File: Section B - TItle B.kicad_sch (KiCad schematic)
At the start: 3 parts, among them IC2 TPS61086DRCR

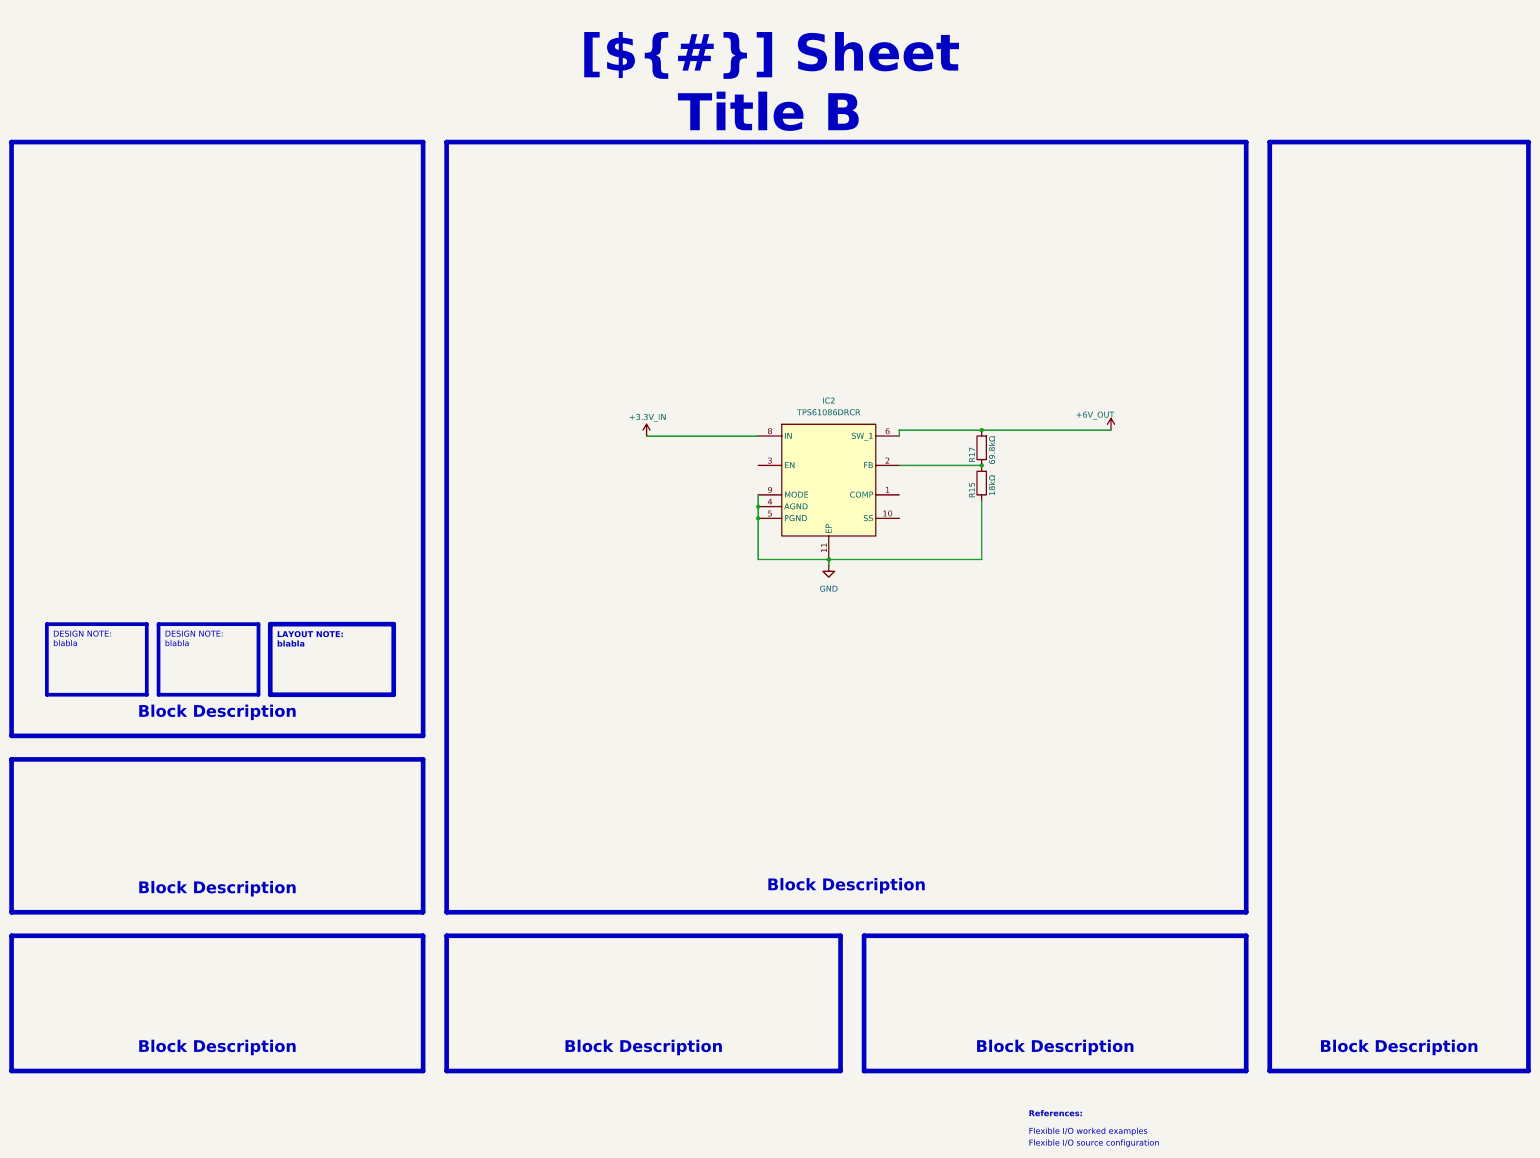
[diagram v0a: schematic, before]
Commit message: [Finish schématique]
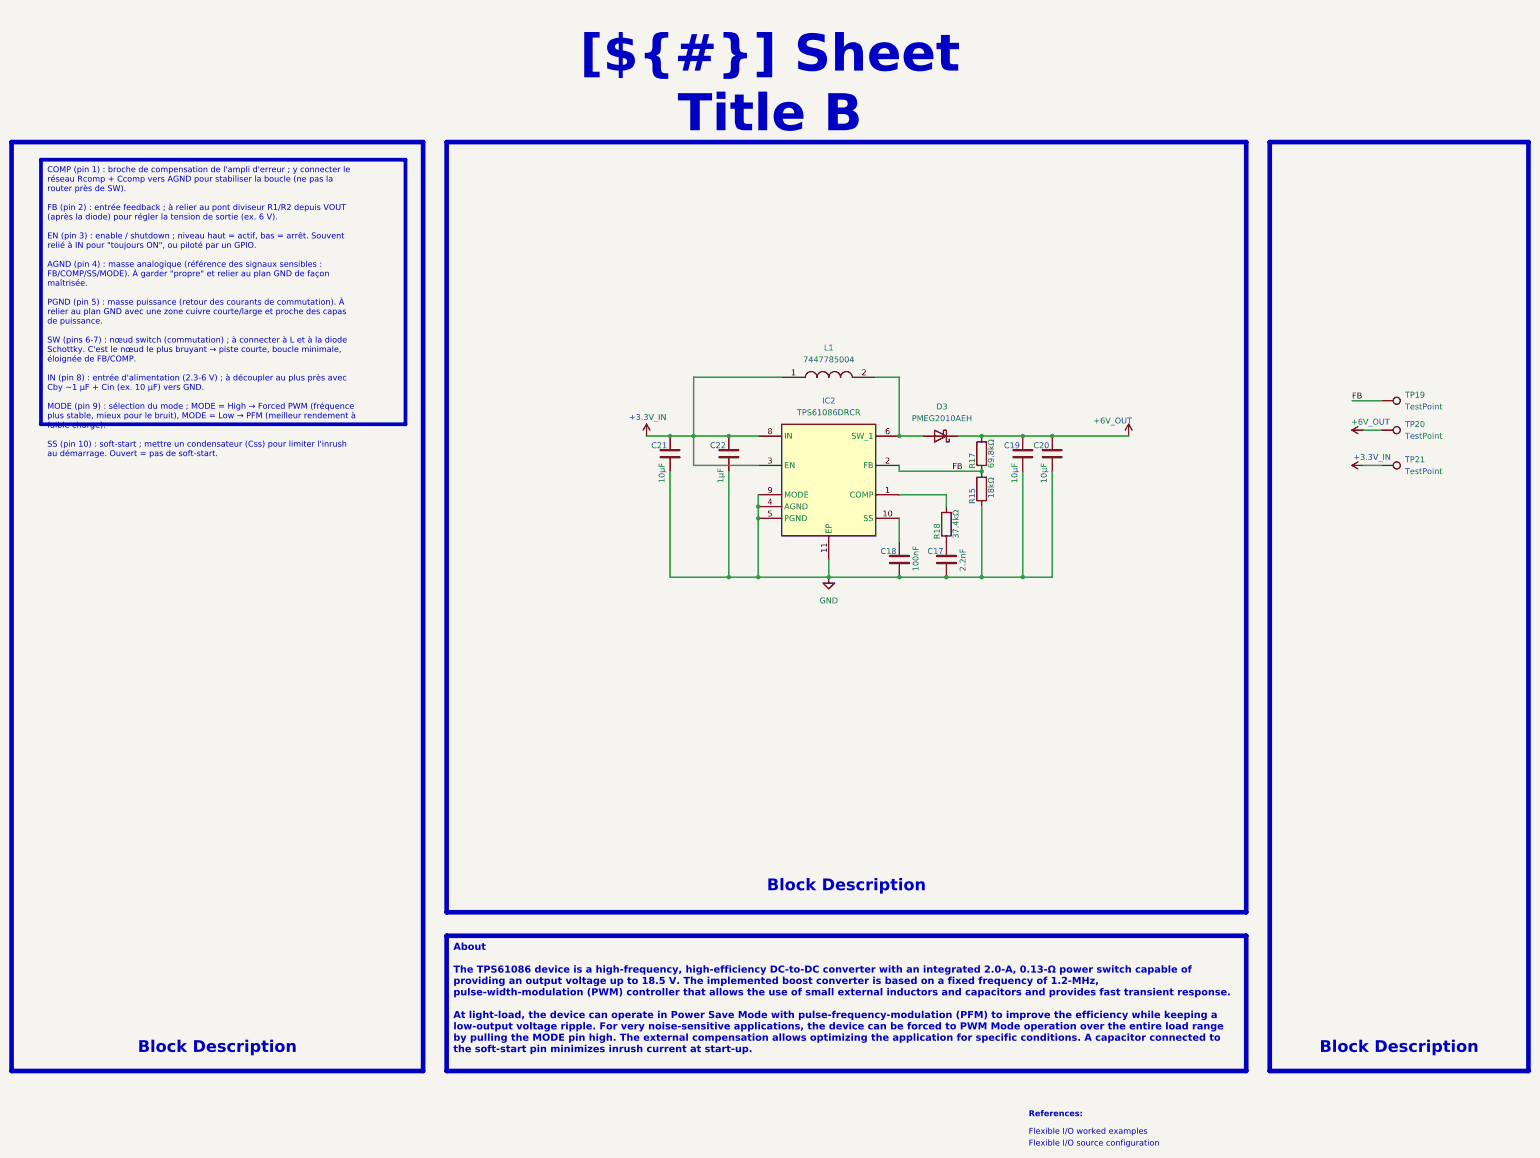
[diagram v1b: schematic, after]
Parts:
- added C17: 2.2nF, Capacitor_SMD:C_0603_1608Metric, symbol Device:C
- added C18: 100nF, Capacitor_SMD:C_0603_1608Metric, symbol Device:C
- added C19, C20, C21: 10µF, Capacitor_SMD:C_0603_1608Metric, symbol Device:C
- added C22: 1µF, Capacitor_SMD:C_0603_1608Metric, symbol Device:C
- added D3: PMEG2010AEH, Diode_SMD:D_SOD-123F, symbol Diode:PMEG2010AEH
- added L1: 7447785004, 7447785004, symbol 7447785004:7447785004
- added R18: 37.4kΩ, Resistor_SMD:R_0603_1608Metric, symbol Device:R
- added TP19, TP20, TP21: TestPoint, TestPoint:TestPoint_Pad_D2.0mm, symbol Connector:TestPoint
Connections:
- net +3.3V_IN: now also IC2.3 (EN), C21.1, C22.1, L1.1, TP21.1
- net +6V_OUT: now also C19.1, C20.1, D3.1 (K), TP20.1; no longer IC2.6 (SW_1), IC2.7 (SW_2)
- net GND: now also C17.2, C18.2, C19.2, C20.2, C21.2, C22.2
- net at IC2.1 (COMP): now also R18.2
- net at IC2.10 (SS): now also C18.1
- net FB: now reaches IC2.2 (FB), R15.2, R17.1
- net FB: now also TP19.1
- new net: C17.1, R18.1
- new net: D3.2 (A), IC2.6 (SW_1), IC2.7 (SW_2), L1.2
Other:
- moved on the sheet: R15, R17

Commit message: [Finish schématiq]
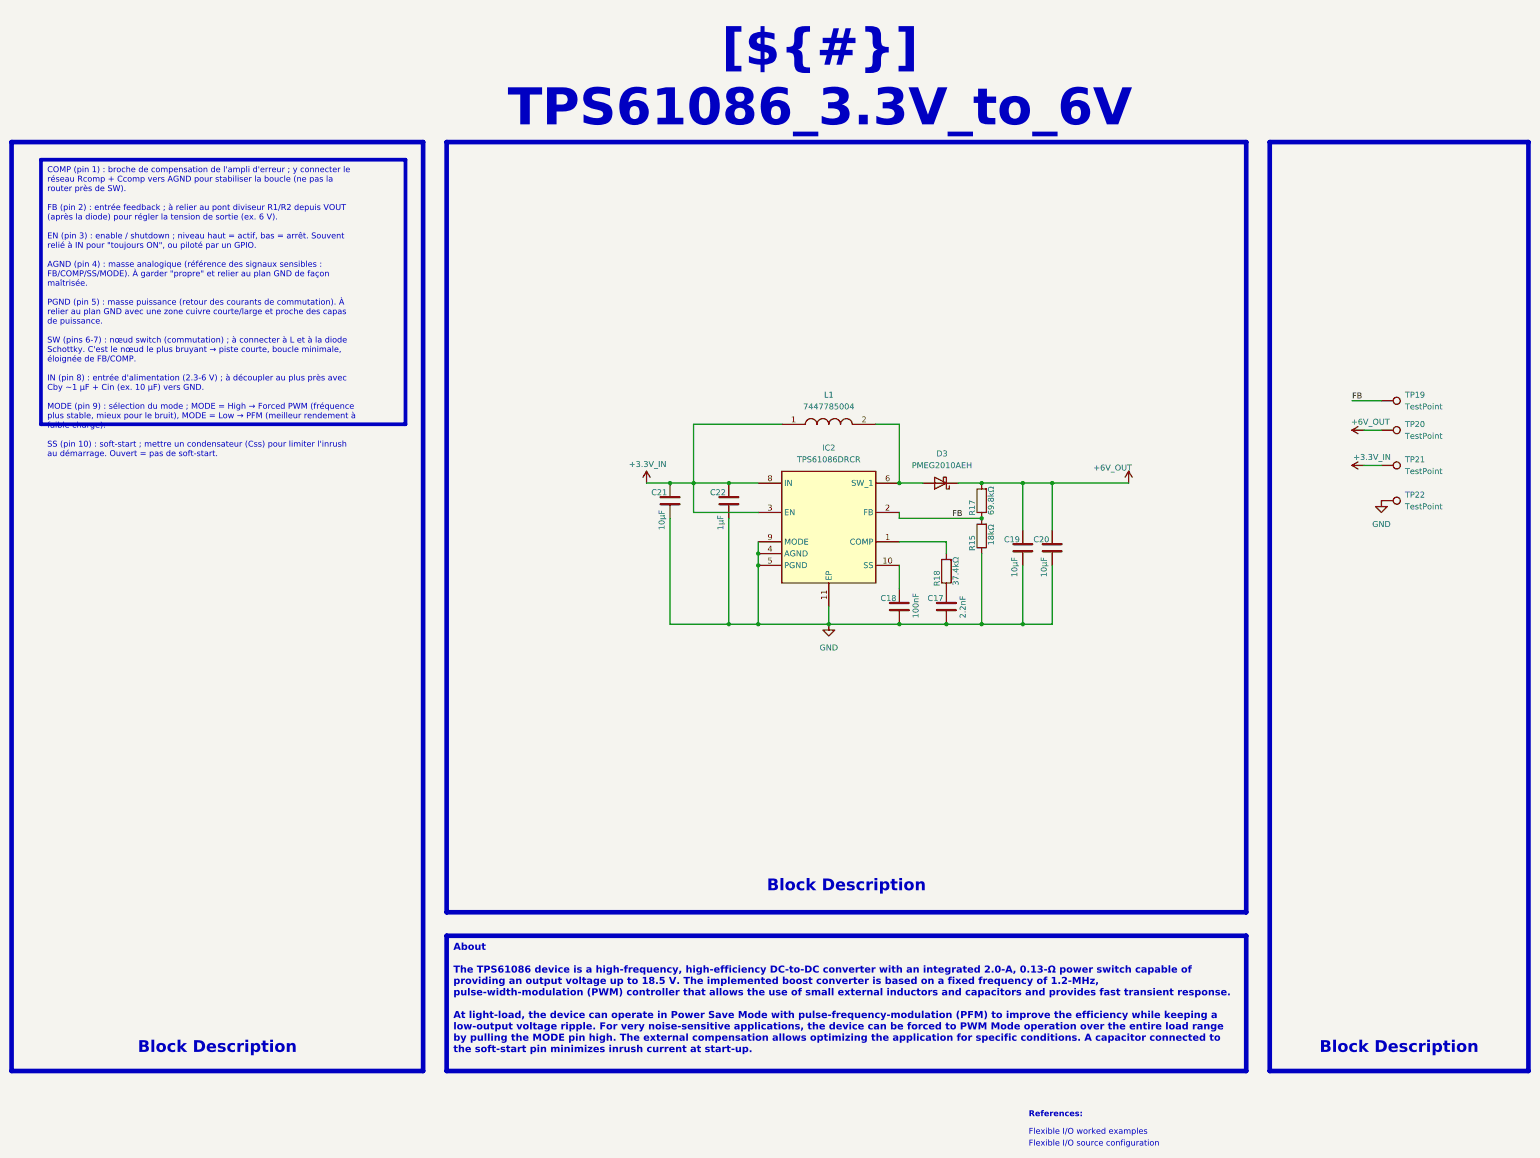
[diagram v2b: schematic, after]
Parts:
- added TP22: TestPoint, TestPoint:TestPoint_Pad_D2.0mm, symbol Connector:TestPoint
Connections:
- net GND: now also TP22.1
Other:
- moved on the sheet: C17, C18, C19, C20, C21, C22, D3, IC2, L1, R15, R17, R18

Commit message: [PCB fini]
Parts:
- L1: footprint 7447785004 -> 7447785004:7447785004
